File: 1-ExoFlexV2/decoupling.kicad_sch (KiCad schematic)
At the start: 158 parts

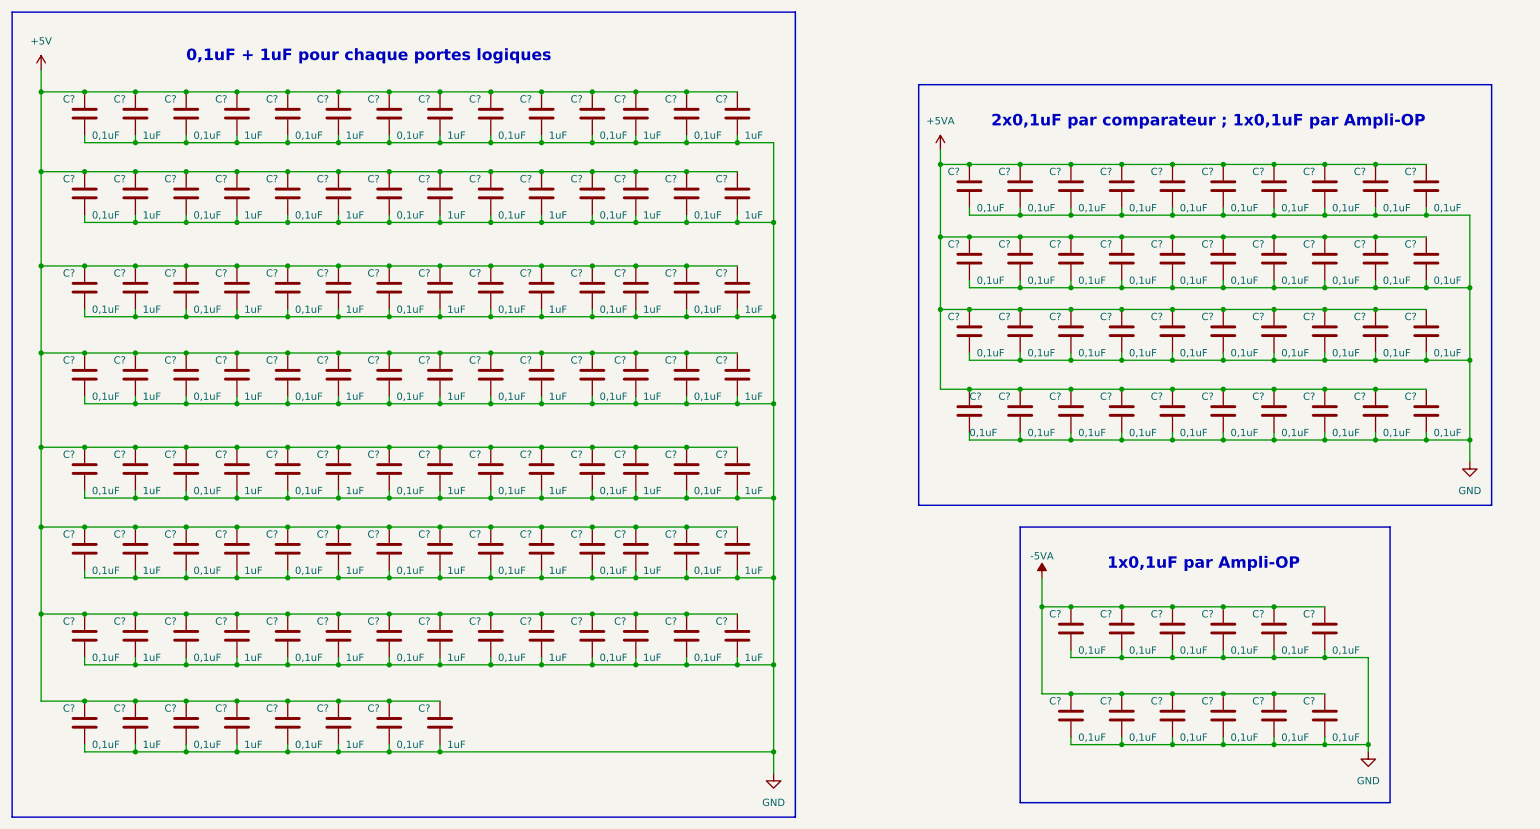
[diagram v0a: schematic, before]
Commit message: Schématisation terminée
- Schéma terminé
- Passage vers le PCB
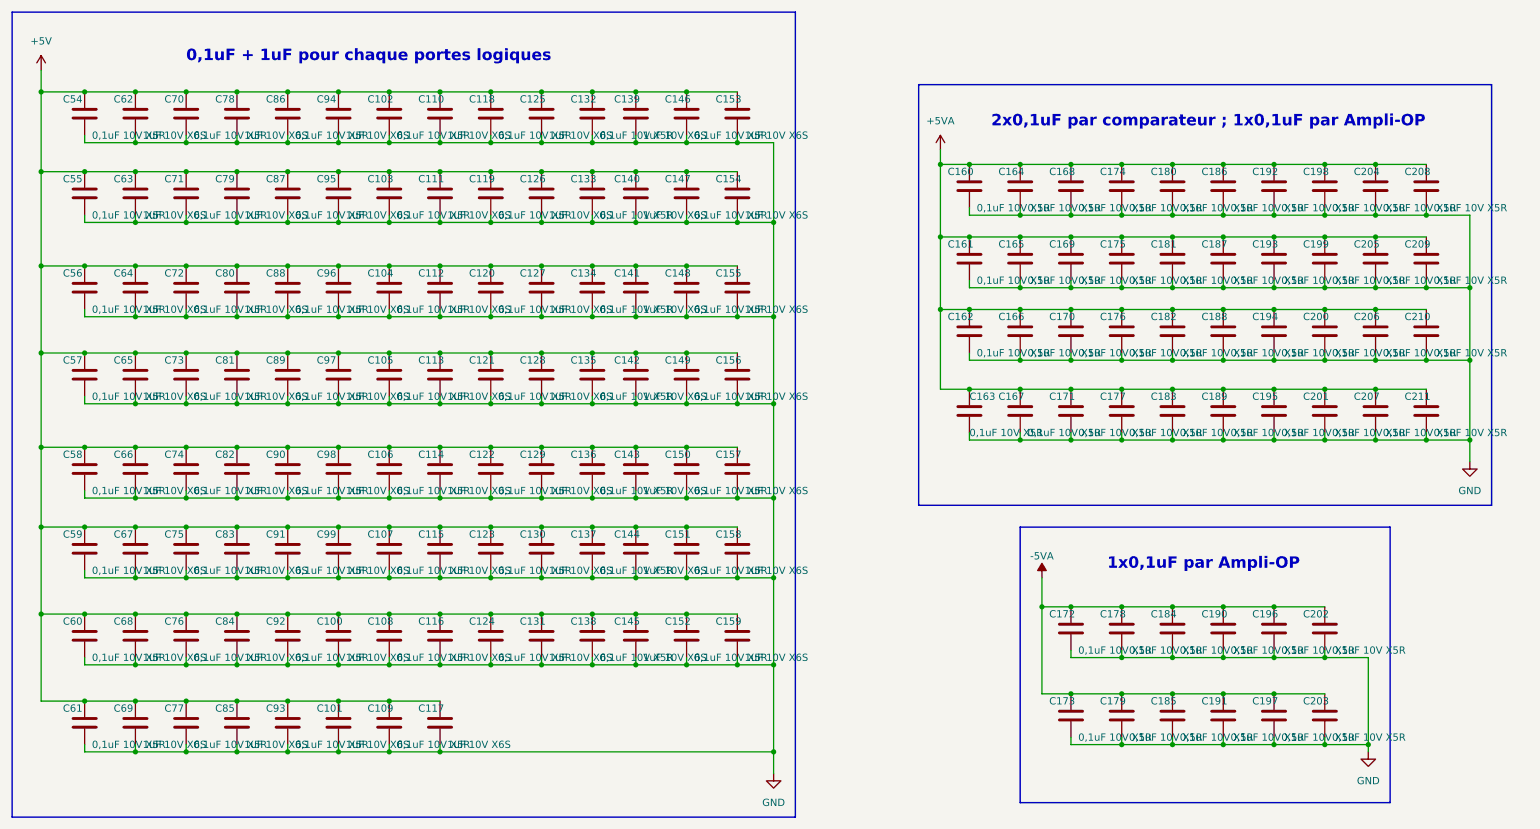
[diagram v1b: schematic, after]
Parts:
- C100, C101, C110, C111, C112, C113, C114, C115, C116, C117, C125, C126, C127, C128, C129, C130, C131, C139, C140, C141, C142, C143, C144, C145, C153, C154, C155, C156, C157, C158, C159, C62, C63, C64, C65, C66, C67, C68, C69, C78, C79, C80, C81, C82, C83, C84, C85, C94, C95, C96, C97, C98, C99: renamed from C?; value 1uF -> 1uF 10V X6S; footprint Capacitor_SMD:C_0603_1608Metric -> Capacitor_SMD:C_0402_1005Metric; DESCRIPTION (none) -> 1 µF ±10% 10V Ceramic Capacitor X6S 0402 (1005 Metric); MANUFACTURER (none) -> Murata Electronics; PACKAGE (none) -> 0402 (1005 Metric); PART NUMBER (none) -> GRM155C81A105KA12D; TYPE (none) -> SMD
- C102, C103, C104, C105, C106, C107, C108, C109, C118, C119, C120, C121, C122, C123, C124, C132, C133, C134, C135, C136, C137, C138, C146, C147, C148, C149, C150, C151, C152, C160, C161, C162, C164, C165, C166, C167, C168, C169, C170, C171, C172, C173, C174, C175, C176, C177, C178, C179, C180, C181, C182, C183, C184, C185, C186, C187, C188, C189, C190, C191, C192, C193, C194, C195, C196, C197, C198, C199, C200, C201, C202, C203, C204, C205, C206, C207, C208, C209, C210, C211, C54, C55, C56, C57, C58, C59, C60, C61, C70, C71, C72, C73, C74, C75, C76, C77, C86, C87, C88, C89, C90, C91, C92, C93: renamed from C?; value 0,1uF -> 0,1uF 10V X5R; footprint Capacitor_SMD:C_0603_1608Metric -> Capacitor_SMD:C_0402_1005Metric; DESCRIPTION (none) -> 0.1 µF ±10% 10V Ceramic Capacitor X5R 0402 (1005 Metric); MANUFACTURER (none) -> Murata Electronics; PACKAGE (none) -> 0402 (1005 Metric); PART NUMBER (none) -> GRM155R61A104KA01D; TYPE (none) -> SMD
- C163: renamed from C?; value 0,1uF -> 0,1uF 10V X5R; footprint FootPrintLib:CAPC220145_88N_KEM -> Capacitor_SMD:C_0402_1005Metric; DESCRIPTION (none) -> 0.1 µF ±10% 10V Ceramic Capacitor X5R 0402 (1005 Metric); MANUFACTURER (none) -> Murata Electronics; PACKAGE (none) -> 0402 (1005 Metric); PART NUMBER (none) -> GRM155R61A104KA01D; TYPE (none) -> SMD
